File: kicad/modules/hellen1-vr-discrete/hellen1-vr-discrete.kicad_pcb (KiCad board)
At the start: 4 copper layers, 15.2 x 9.8 mm, 45 parts, among them M750 Module-vr-discrete-0.1, U751 SRV05-4-P-T7, U752 74AHC1G02, U753 MCP6004, U754 MAX9142, U755 NC7SB3157P6X, U756 NC7SB3157P6X, U757 74AHC1G02

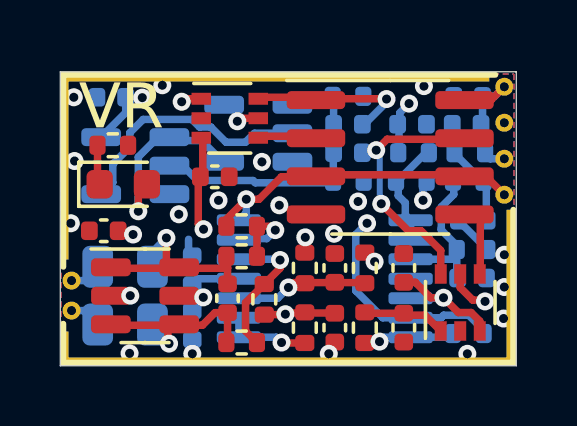
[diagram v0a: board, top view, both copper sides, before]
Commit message: add VR 0.2
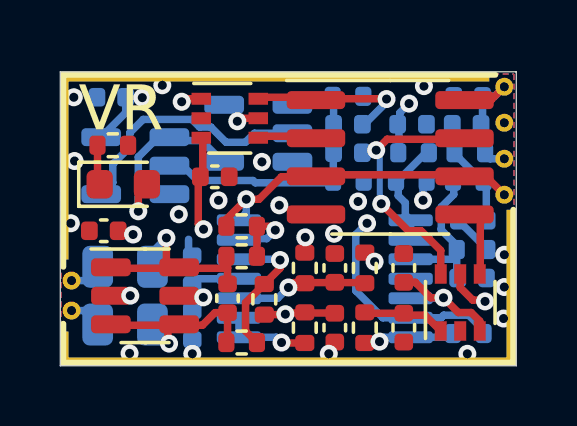
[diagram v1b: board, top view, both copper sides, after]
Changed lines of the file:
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@@
   (gr_rect (start 77.7 95.05) (end 92.9 85.25) (layer "Edge.Cuts") (width 0.02) (fill none))
   (gr_rect (start 77.7 95.05) (end 92.9 85.25) (layer "User.1") (width 0.02) (fill none))
-  (gr_text "VR" (at 79.735274 86.410274) (layer "F.SilkS")
+  (gr_text "VR" (at 79.724999 86.475135) (layer "F.SilkS")
     (effects (font (size 1.5 1.5) (thickness 0.2)))
   )
@@
   (segment (start 82.342385 87.092385) (end 82.089116 86.839116) (width 0.25) (layer "B.Cu") (net 29))
   (segment (start 85.6375 87.3) (end 84.169298 87.3) (width 0.25) (layer "B.Cu") (net 29))
+  (zone (net 0) (net_name "") (layers "F.Cu" "In1.Cu" "In2.Cu" "B.Cu") (hatch edge 0.508)
+    (connect_pads (clearance 0))
+    (min_thickness 0.254)
+    (keepout (tracks allowed) (vias allowed) (pads allowed) (copperpour not_allowed) (footprints allowed))
+    (fill (thermal_gap 0.508) (thermal_bridge_width 0.508))
+    (polygon
+      (pts
+        (xy 92.85 89.35)
+        (xy 92.2 89.35)
+        (xy 92.2 85.325)
+        (xy 92.825 85.325)
+      )
+    )
+  )
   (zone (net 1) (net_name "GND") (layers "F.Cu" "In1.Cu" "In2.Cu" "B.Cu") (hatch edge 0.508)
     (connect_pads (clearance 0))
